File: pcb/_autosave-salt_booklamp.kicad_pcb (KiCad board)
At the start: 2 copper layers, 45.1 x 45.1 mm, 28 parts, among them J1 USB-C31-S-RA-CS1E-BK-T/R, P1 PIC-TC2050-IDC, U1 PIC16F15213-I/SN, U2 BQ21040DBVR, U3 TPS61158DRVR

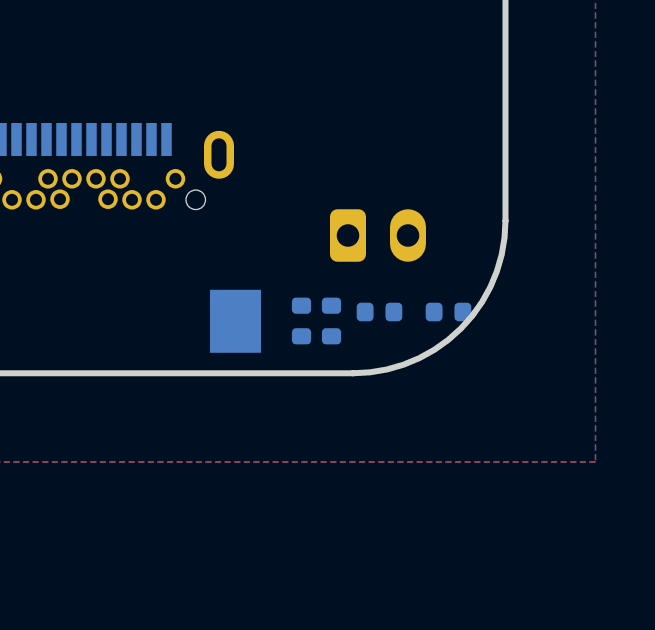
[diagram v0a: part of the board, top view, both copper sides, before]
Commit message: Work on placement for pcb .step transfer
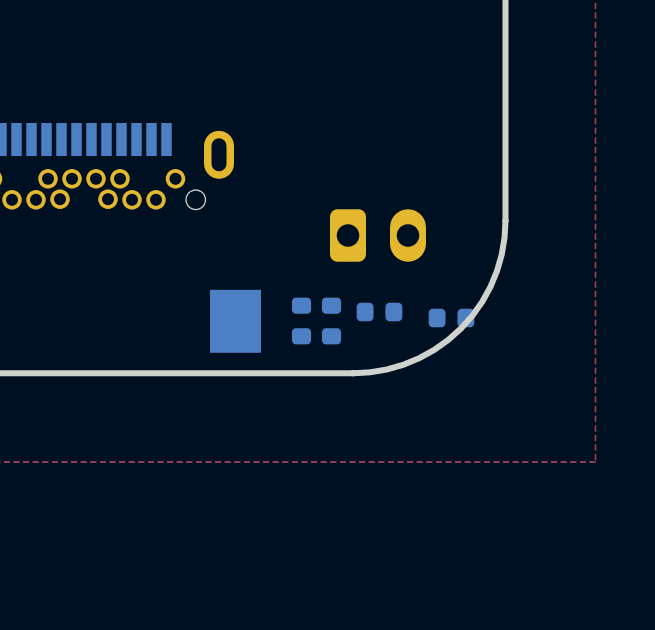
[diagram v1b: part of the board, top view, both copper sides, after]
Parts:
- moved C2 0.22 mm to (245.0, 149.7)
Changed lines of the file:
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@@
 	(footprint "Capacitor_SMD:C_0402_1005Metric"
 		(layer "B.Cu")
-		(at 244.882 149.532 180)
+		(at 244.982 149.732 180)
 		(descr "Capacitor SMD 0402 (1005 Metric), square (rectangular) end terminal, IPC_7351 nominal, (Body size source: IPC-SM-782 page 76, https://www.pcb-3d.com/wordpress/wp-content/uploads/ipc-sm-782a_amendment_1_and_2.pdf), generated with kicad-footprint-generator")
 		(tags "capacitor")
